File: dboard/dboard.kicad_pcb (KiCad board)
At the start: 2 copper layers, 49 x 11 mm, 10 parts, among them J1 Conn_01x04, U1 SRV05-4

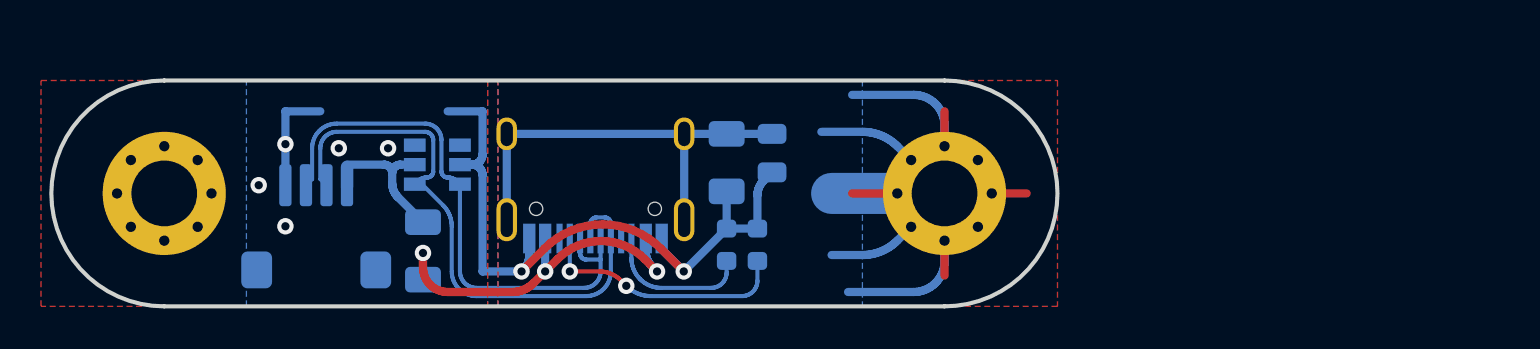
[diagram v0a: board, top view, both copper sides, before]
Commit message: Add all the shit lmao
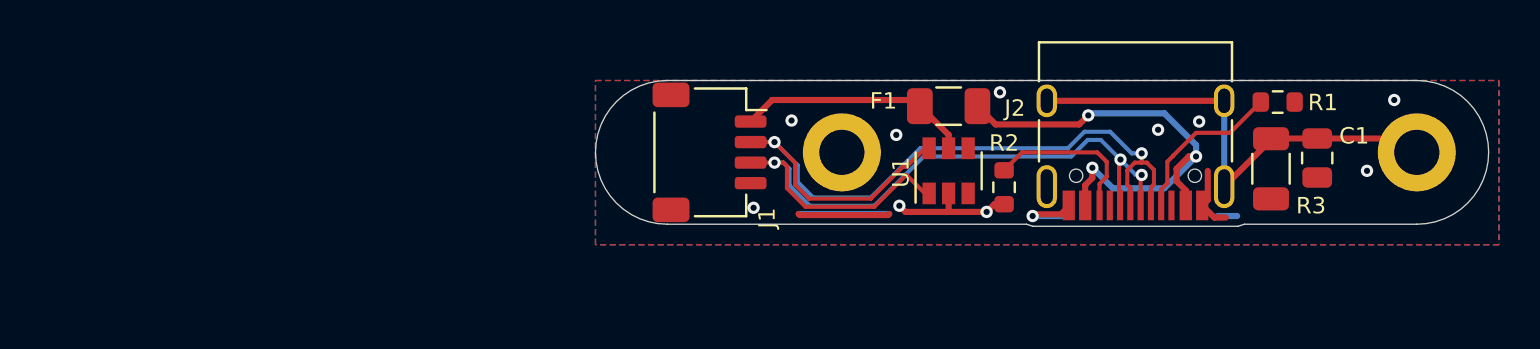
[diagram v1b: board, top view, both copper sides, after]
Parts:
- removed USB1: HRO-TYPE-C-31-M-12, Type-C:HRO-TYPE-C-31-M-12-Assembly
- added J2: USB_C_Receptacle_USB2.0, Connector_USB:USB_C_Receptacle_HRO_TYPE-C-31-M-12, F.Cu at (26.3, 2.04)
- added Ref**: Val**, pcbart:tt_4mm, F.Cu at (3.90, 3.60)
- C1, F1, R1, R2, R3, U1: moved to F.Cu
- H1: footprint crokto:M3_Via_Hole_NC -> MountingHole:MountingHole_2.2mm_M2_DIN965_Pad
- H2: footprint crokto:M3_Via_Hole -> MountingHole:MountingHole_2.2mm_M2_DIN965_Pad
- J1: value Conn_01x04 -> JST_SH_SM04B-SRSS-TB_1x04; footprint crokto:JST_SH_SM04B-SRSS-TB_1x04-1MP_P1.00mm_Horizontal -> Connector_JST:JST_SH_SM04B-SRSS-TB_1x04-1MP_P1.00mm_Horizontal; moved to F.Cu
- moved H1 33.1 mm to (12.0, 3.50)
- moved F1 26.6 mm to (17.2, 1.25), turned to 0 degrees
- moved C1 26.6 mm to (35.1, 3.77)
- moved R3 26.5 mm to (32.9, 4.30)
- moved R1 26.3 mm to (33.2, 1.05), turned to 180 degrees
- moved U1 24.9 mm to (17.2, 4.40), turned to 90 degrees
- moved H2 23.1 mm to (40.0, 3.50)
- moved J1 19.5 mm to (5.56, 3.50), turned to -90 degrees
- moved R2 13.8 mm to (19.9, 5.20), turned to 90 degrees
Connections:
- J1 pad 2: D+ -> D-
- J1 pad 3: D- -> D+
- U1 pad 1: (no net) -> D+
- U1 pad 3: D- -> unconnected-(U1-Pad3)
- U1 pad 4: D+ -> unconnected-(U1-Pad4)
- U1 pad 6: (no net) -> D-
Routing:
- net SHIELD: track 74.6 -> 23.7 mm
- net GND: track 40.3 -> 22.5 mm, vias 7 -> 11
- net D-: track 27.6 -> 38.3 mm, vias 0 -> 2
- net D+: track 29.5 -> 36.2 mm, vias 0 -> 3
- net VBUS: track 18.8 -> 23.8 mm
- net Net-(J2-PadA5): track 12.5 -> 8.06 mm, vias 2 -> 0
- net +5V: track 7.74 -> 11.0 mm
- removed copper zone on B.Cu, net SHIELD
- removed copper zone on F.Cu, net SHIELD
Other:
- board size 49 x 11 mm -> 43.5 x 7.1 mm
- net class Default removed
- net class Power removed
- rule pad_to_mask_clearance: 0.051 -> 0
- board text added: "TapTap DB"
